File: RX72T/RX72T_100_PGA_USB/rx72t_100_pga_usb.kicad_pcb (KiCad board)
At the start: 2 copper layers, 109 parts, among them J1 DA_OUT, J10 EMU_MODE, J11 SCI1, J12 5V_POW, J13 12V_POW, J14 CAN, J15 Micro_SD_Card_Det_Hirose_DM3AT, J16 SLAVE, J17 MASTER, J18 I2C_B, J19 I2C_A, J2 GPTW_012, J20 RSPI, J21 SCI8, J22 SCI11, J23 SPI8, J24 SPI11, J25 RS-485 TERM, J26 RS-485, J27 MD, J28 SER/RS-485, J29 5VIN, J3 GPTW_456, J4 EXT_DG0, J5 EXT_AN, J6 SCI1_POW, J7 UB, J8 EXT_DG1, J9 E1_E2_Lite, M1 BP5293-5, SW2 RESET, U1 NJU7223DL1-33, U2 SN65HVD230, U3 MIC2026-1BM, U4 MIC2026-1BM, U5 MAX3485, U6 RX72T_100_PGA_USB, X1 16MHz

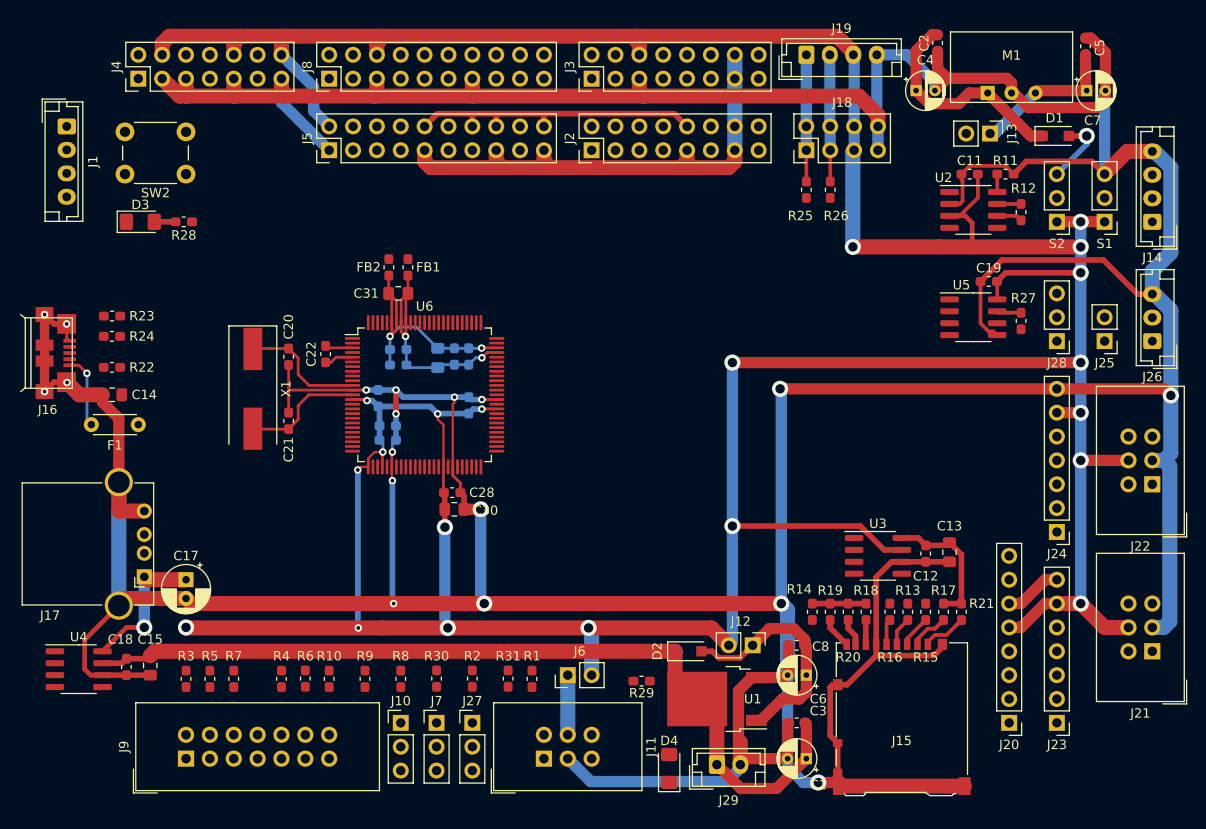
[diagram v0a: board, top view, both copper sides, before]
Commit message: Update: cleanup
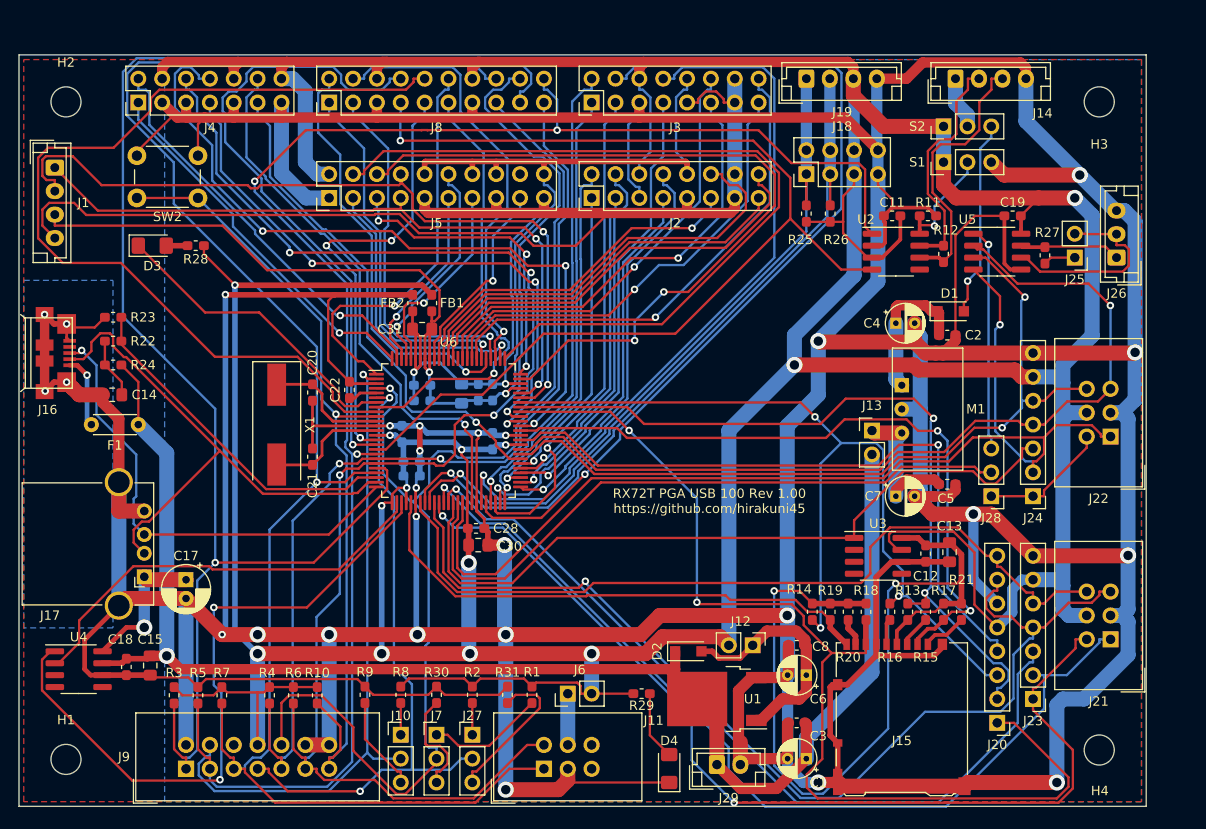
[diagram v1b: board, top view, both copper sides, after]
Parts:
- added H1: Hole, MountingHole:MountingHole_3.2mm_M3, F.Cu at (55.0, 145.0)
- added H2: Hole, MountingHole:MountingHole_3.2mm_M3, F.Cu at (55.0, 75.0)
- added H3: Hole, MountingHole:MountingHole_3.2mm_M3, F.Cu at (165.0, 75.0)
- added H4: Hole, MountingHole:MountingHole_3.2mm_M3, F.Cu at (165.0, 144.0)
- J15: value Micro_SD_Card_Det_Hirose_DM3AT -> MSD_Hirose_DM3AT
- moved C5 48.9 mm to (148.8, 115.7), turned to 180 degrees
- moved C7 47.7 mm to (143.3, 117.0)
- moved M1 35.6 mm to (144.0, 107.7), turned to 270 degrees
- moved J13 34.0 mm to (140.8, 110.0), turned to 0 degrees
- moved C2 31.1 mm to (148.8, 99.8), turned to 180 degrees
- moved J14 25.9 mm to (149.7, 72.5), turned to 0 degrees
- moved C4 24.9 mm to (143.3, 98.6)
- moved D1 21.8 mm to (149.2, 97.3)
- moved S1 18.3 mm to (148.4, 81.4), turned to 90 degrees
- moved J28 17.9 mm to (153.5, 117.0)
- moved S2 15.8 mm to (148.4, 77.6), turned to 90 degrees
- moved J26 9.67 mm to (166.8, 91.6)
- moved J25 9.44 mm to (162.4, 91.6)
- moved C11 9.38 mm to (142.9, 87.1)
- moved R11 9.38 mm to (146.8, 87.1)
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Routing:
- net GND: track 682.8 -> 950.1 mm, vias 18 -> 27
- net /PD3: track 0.00 -> 178.6 mm, vias 0 -> 1
- net /PD7: track 0.00 -> 176.7 mm, vias 0 -> 3
- net /PD4: track 0.00 -> 160.7 mm, vias 0 -> 1
- net +3V3: track 446.0 -> 598.3 mm, vias 20 -> 13
- net /PD5: track 0.00 -> 136.6 mm, vias 0 -> 2
- net /P00: track 0.00 -> 131.1 mm, vias 0 -> 1
- net /PE0: track 0.00 -> 116.8 mm, vias 0 -> 1
- net /RX72T/PA0_TXD11: track 0.00 -> 113.8 mm, vias 0 -> 1
- net /I2C_SPI_SCI/PB0: track 0.00 -> 111.8 mm, vias 0 -> 1
- net /I2C_SPI_SCI/MISO: track 2.60 -> 113.2 mm, vias 0 -> 2
- net /RX72T/PA5_RXD8: track 0.00 -> 105.5 mm, vias 0 -> 2
- net /PD6: track 0.00 -> 103.0 mm, vias 0 -> 2
- net /RX72T/PA4_TXD8: track 0.00 -> 98.9 mm, vias 0 -> 1
- net /PE3: track 0.00 -> 98.3 mm
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- added copper zone on B.Cu, net +3V3
- added copper zone on B.Cu, net GND
- added copper zone on F.Cu, net GND
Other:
- board outline added: 120 x 80 mm
- board text added: "RX72T PGA USB 100 Rev 1.00 https://github.com/hirakuni45"

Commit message: Update: cleanup
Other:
- net class Default removed
